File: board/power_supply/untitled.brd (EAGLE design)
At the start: 52 x 55 mm, 27 parts, among them IC1 317EMP, Q1 FDD4141TO252

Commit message: update boards 2022-07-14
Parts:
- C1: value (none) -> 22uF 25V
- C2: value (none) -> 10uF 10V
- C3, C4: value (none) -> 0.1uF
- R1: value (none) -> 300Ω
- R2: value (none) -> 470kΩ
- R3: value (none) -> 20kΩ
- R4: value (none) -> 1.2kΩ
- R6: value (none) -> 1.2KΩ 1/6W
- R7: value 10k -> 300Ω
- U$2: value SMD-R-TRIM -> 2.2kΩ
- U$4: value R-TRIM -> 20kΩ
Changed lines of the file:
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@@
 <?xml version="1.0" encoding="utf-8"?>
 <!DOCTYPE eagle SYSTEM "eagle.dtd">
-<eagle version="9.6.1">
+<eagle version="9.6.2">
 <drawing>
 <settings>
-<setting alwaysvectorfont="yes"/>
+<setting alwaysvectorfont="no"/>
 <setting verticaltext="up"/>
 </settings>
@@
 </layers>
 <board>
-<fusionsync huburn="a.cGVyc29uYWw6dWUyYjhiNWJj" projecturn="a.cGVyc29uYWw6dWUyYjhiNWJjIzIwMjIwNDE2NTE3MzEzNjU2" f3durn="urn:adsk.wipprod:dm.lineage:QmnGeXTNRAeKhx4INCeYVg" pcbguid="" lastpulledtime="" lastsyncedchangeguid="" latestrevisionid="b83a574e-0160-4f8e-8456-9f8577d503a8" lastsyncedrevisionid="b83a574e-0160-4f8e-8456-9f8577d503a8" lastboardhashguid="a0df0de1-b480-8f0f-8af4-34f871867293" lastpushedtime="2022-07-09T12:07:00Z" linktopcb3d="%12"/>
+<fusionsync huburn="a.cGVyc29uYWw6dWUyYjhiNWJj" projecturn="a.cGVyc29uYWw6dWUyYjhiNWJjIzIwMjIwNDE2NTE3MzEzNjU2" f3durn="urn:adsk.wipprod:dm.lineage:QmnGeXTNRAeKhx4INCeYVg" pcbguid="" lastpulledtime="" lastsyncedchangeguid="" latestrevisionid="b83a574e-0160-4f8e-8456-9f8577d503a8" lastsyncedrevisionid="b83a574e-0160-4f8e-8456-9f8577d503a8" lastboardhashguid="a0df0de1-b480-8f0f-8af4-34f871867293" lastpushedtime="2022-07-09T12:07:00Z" linktopcb3d="true"/>
 <plain>
 <wire x1="51.943" y1="-2.254" x2="51.943" y2="48.746" width="0.001" layer="20"/>
@@
 <attribute name="VALUE" x="3.81" y="12.63" size="0.0254" layer="27"/>
 </element>
-<element name="R1" library="adafruit" package="M2012" value="" x="31.75" y="15.748" smashed="yes">
+<element name="R1" library="adafruit" package="M2012" value="300Ω" x="31.75" y="15.748" smashed="yes">
 <attribute name="NAME" x="27.432" y="15.24" size="1.27" layer="25"/>
 <attribute name="VALUE" x="30.734" y="13.462" size="1.27" layer="27"/>
 </element>
-<element name="U$2" library="by_hirame" package="SMD-R-TRIM" value="SMD-R-TRIM" x="31.75" y="19.05" smashed="yes"/>
+<element name="U$2" library="by_hirame" package="SMD-R-TRIM" value="2.2kΩ" x="31.75" y="19.05" smashed="yes"/>
 <element name="MD1" library="Rembrandt Electronics - JST XH Connectors v1-0" package="JST-XH-02-PACKAGE-LONG-PAD" value="JST-XH-02-PIN-LONG-PAD" x="46.101" y="22.098" smashed="yes" rot="R270">
 <attribute name="NAME" x="43.37" y="20.82" size="1.016" layer="25" ratio="10" rot="R90"/>
@@
 <attribute name="PURCHASE-URL" value="https://pricing.snapeda.com/search/part/OKL-T/6-W12P-C/?ref=eda" x="21.209" y="37.846" size="1.778" layer="27" rot="R180" display="off"/>
 </element>
-<element name="R3" library="adafruit" package="M2012" value="" x="20.955" y="30.226" smashed="yes">
+<element name="R3" library="adafruit" package="M2012" value="20kΩ" x="20.955" y="30.226" smashed="yes">
 <attribute name="NAME" x="22.987" y="29.591" size="1.27" layer="25"/>
 <attribute name="VALUE" x="19.939" y="27.94" size="1.27" layer="27"/>
 </element>
-<element name="C1" library="adafruit" package="C2012" value="" x="20.955" y="28.067" smashed="yes" rot="R180">
+<element name="C1" library="adafruit" package="C2012" value="22uF 25V" x="20.955" y="28.067" smashed="yes" rot="R180">
 <attribute name="NAME" x="25.4" y="28.702" size="1.27" layer="25" rot="R180"/>
 <attribute name="VALUE" x="21.844" y="30.353" size="1.27" layer="27" rot="R180"/>
 </element>
-<element name="R4" library="adafruit" package="M2012" value="" x="8.255" y="30.226" smashed="yes">
+<element name="R4" library="adafruit" package="M2012" value="1.2kΩ" x="8.255" y="30.226" smashed="yes">
 <attribute name="NAME" x="7.239" y="27.813" size="1.27" layer="25"/>
 <attribute name="VALUE" x="7.239" y="27.94" size="1.27" layer="27"/>
 </element>
-<element name="C2" library="adafruit" package="C2012" value="" x="13.589" y="27.94" smashed="yes">
+<element name="C2" library="adafruit" package="C2012" value="10uF 10V" x="13.589" y="27.94" smashed="yes">
 <attribute name="NAME" x="15.748" y="27.305" size="1.27" layer="25"/>
 <attribute name="VALUE" x="12.7" y="25.654" size="1.27" layer="27"/>
 </element>
-<element name="R6" library="adafruit" package="0805-THM" value="" x="12.7" y="35.56" smashed="yes" rot="R270">
+<element name="R6" library="adafruit" package="0805-THM" value="1.2KΩ  1/6W" x="12.7" y="35.56" smashed="yes" rot="R270">
 <attribute name="NAME" x="14.224" y="38.608" size="1.27" layer="25" ratio="10" rot="R270"/>
 <attribute name="VALUE" x="9.925" y="38.6906" size="1.27" layer="27" ratio="10" rot="R270"/>
@@
 <attribute name="VALUE" x="24.13" y="7.6708" size="1.27" layer="27" rot="R180"/>
 </element>
-<element name="C3" library="generic" package="SMD1608" value="" x="21.59" y="11.684" smashed="yes">
+<element name="C3" library="generic" package="SMD1608" value="0.1uF" x="21.59" y="11.684" smashed="yes">
 <attribute name="NAME" x="20.79" y="12.334" size="1.016" layer="25"/>
 <attribute name="VALUE" x="20.79" y="10.034" size="1.016" layer="27"/>
 </element>
-<element name="C4" library="generic" package="SMD1608" value="" x="25.146" y="2.413" smashed="yes">
+<element name="C4" library="generic" package="SMD1608" value="0.1uF" x="25.146" y="2.413" smashed="yes">
 <attribute name="NAME" x="24.346" y="3.063" size="1.016" layer="25"/>
 <attribute name="VALUE" x="24.346" y="0.763" size="1.016" layer="27"/>
 </element>
-<element name="R2" library="adafruit" package="M2012" value="" x="31.75" y="13.462" smashed="yes" rot="R180">
+<element name="R2" library="adafruit" package="M2012" value="470kΩ" x="31.75" y="13.462" smashed="yes" rot="R180">
 <attribute name="NAME" x="29.718" y="14.097" size="1.27" layer="25" rot="R180"/>
 <attribute name="VALUE" x="32.766" y="15.748" size="1.27" layer="27" rot="R180"/>
 </element>
-<element name="U$4" library="by_hirame" package="R-TRIM" value="R-TRIM" x="8.128" y="36.703" smashed="yes" rot="R270"/>
+<element name="U$4" library="by_hirame" package="R-TRIM" value="20kΩ" x="8.128" y="36.703" smashed="yes" rot="R270"/>
 <element name="R5" library="adafruit" package="M2012" value="10k" x="28.448" y="10.033" smashed="yes" rot="R180">
 <attribute name="NAME" x="29.464" y="9.017" size="1.27" layer="25" rot="R180"/>
 <attribute name="VALUE" x="29.464" y="12.319" size="1.27" layer="27" rot="R180"/>
 </element>
-<element name="R7" library="adafruit" package="M2012" value="10k" x="28.448" y="5.08" smashed="yes">
+<element name="R7" library="adafruit" package="M2012" value="300Ω" x="28.448" y="5.08" smashed="yes">
 <attribute name="NAME" x="27.432" y="6.096" size="1.27" layer="25"/>
 <attribute name="VALUE" x="27.432" y="2.794" size="1.27" layer="27"/>

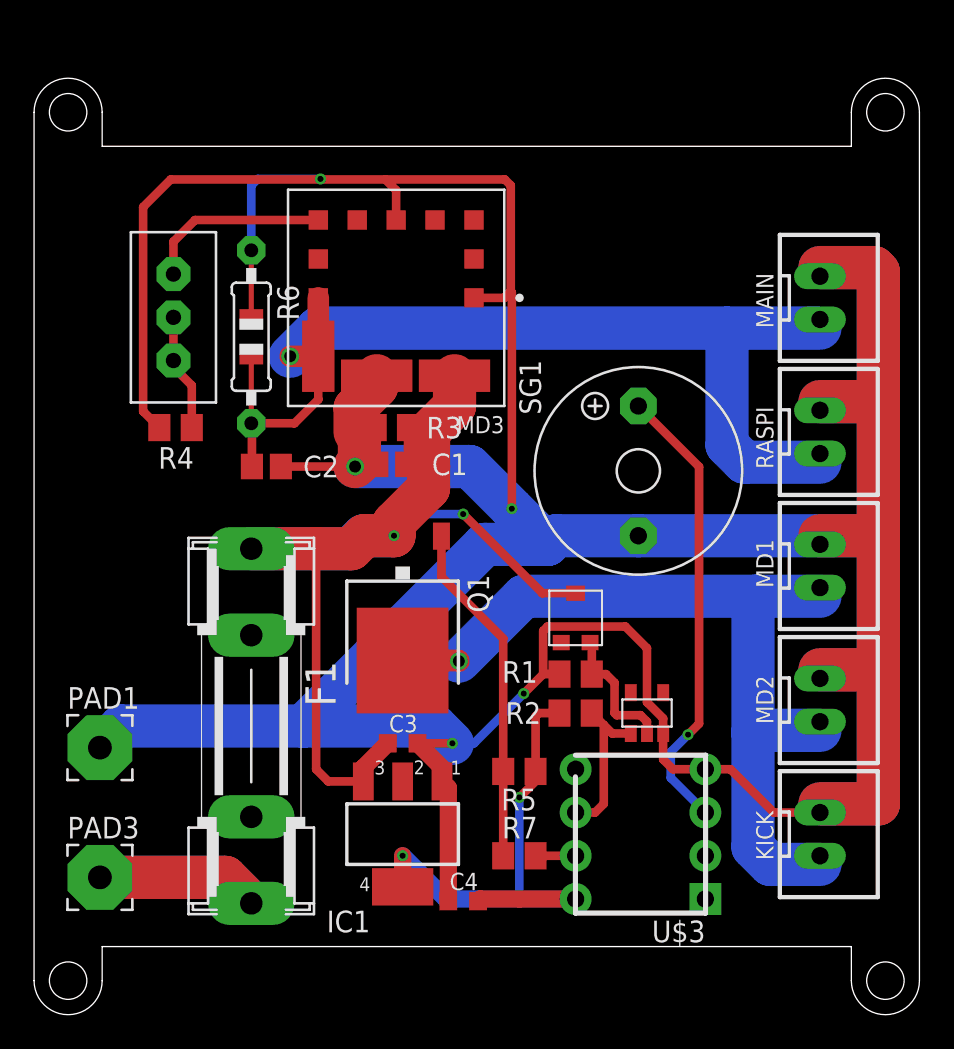
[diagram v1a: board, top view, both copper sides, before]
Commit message: marge前のファイル
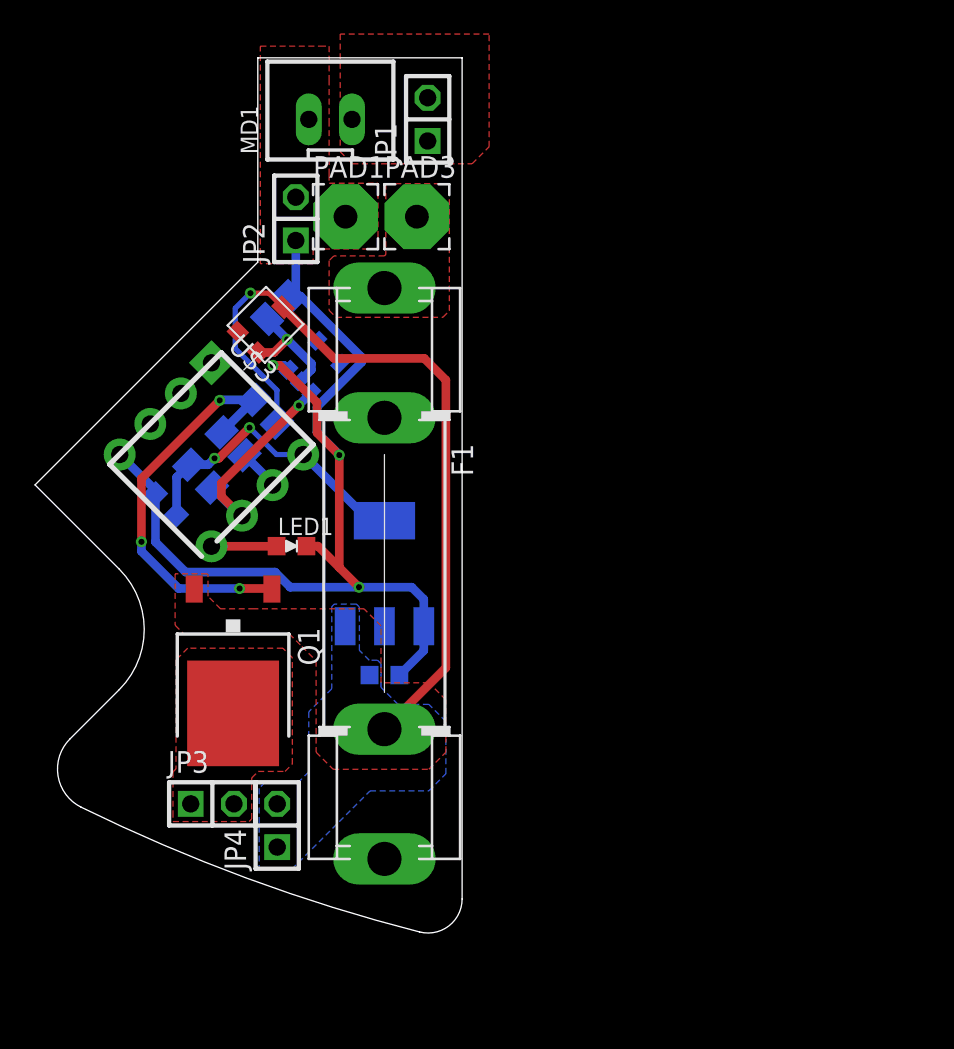
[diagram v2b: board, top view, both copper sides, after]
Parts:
- removed C1: 22uF 25V, adafruit:C2012
- removed C2: 10uF 10V, adafruit:C2012
- removed KICK, MAIN, MD2, RASPI: JST-XH-02-PIN-LONG-PAD, Rembrandt Electronics - JST XH Connectors v1-0:JST-XH-02-PACKAGE-LONG-PAD
- removed MD3: OKL-T/6-W12P-CMURATA_OKL-T-6-W12P-C_0_0, OKL-T_6-W12P-C:MURATA_OKL-T-6-W12P-C_0
- removed R3: 20kΩ, adafruit:M2012
- removed R4: 1.2kΩ, adafruit:M2012
- removed R6: 1.2KΩ 1/6W, adafruit:0805-THM
- removed SG1: F/TMB, buzzer:F/TMB
- removed U$4: 20kΩ, by_hirame:R-TRIM
- added JP1, JP2, JP3, JP4: (no value), pinhead:1X02
- added LED1: LED1608, generic:LED1608
- F1: device fuse:SHK20L -> fuse:SH32
- moved PAD3 43.0 mm to (22.4, 42.6)
- moved MD1 38.9 mm to (17.3, 48.3), turned to 0 degrees
- moved PAD1 34.4 mm to (18.2, 42.6)
- moved U$3 33.6 mm to (10.4, 28.6), turned to 315 degrees
- moved R7 29.5 mm to (11.6, 29.3), flipped to the bottom, turned to 225 degrees
- moved C4 29.1 mm to (7.69, 25.7), flipped to the bottom, turned to 225 degrees
- moved U$1 28.2 mm to (16.4, 33.8), flipped to the bottom, turned to 45 degrees
- moved R1 27.7 mm to (14.3, 37.3), flipped to the bottom, turned to 315 degrees
- moved R2 26.1 mm to (9.73, 27.4), flipped to the bottom, turned to 45 degrees
- moved R5 25.9 mm to (13.5, 31.2), flipped to the bottom, turned to 45 degrees
- moved U$2 25.1 mm to (13.5, 36.3), turned to 315 degrees
- moved IC1 15.3 mm to (20.5, 21.7), flipped to the bottom, turned to 0 degrees
- moved F1 11.9 mm to (20.5, 21.7)
- moved Q1 10.4 mm to (11.6, 15.9)
- moved C3 4.15 mm to (20.5, 15.7), flipped to the bottom, turned to 180 degrees
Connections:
- removed net N$8: C2.1, MAIN.2, MD3.4, MD3.5, R6.2, RASPI.2
- removed net N$9: MD3.6, U$4.P$1
- net GND: now also JP2.1, JP2.2, LED1.K; no longer C1.2, C2.2, KICK.1, MAIN.1, MD2.1, MD3.1, MD3.3, MD3.7, R3.1, R4.1, R6.1, RASPI.1, SG1.-
- net N$11: no longer R5.1
- net N$3: now also F1.1A; no longer F1.2A
- net N$5: now also JP3.1, JP3.2; no longer KICK.2, MD1.2, MD2.2
- net N$6: now also LED1.A, U$3.5; no longer SG1.+, U$3.3
- net N$7: now also JP1.1, JP1.2, MD1.2; no longer R4.2, U$4.P$2, U$4.P$3
- net VCC: now also F1.2A, JP4.1, JP4.2, R5.1; no longer C1.1, F1.1A, MD3.2, R3.2
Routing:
- net GND: track 301.2 -> 63.5 mm, vias 5 -> 3
- net N$8: track 60.2 -> 0.00 mm, vias 1 -> 0
- net N$5: track 50.8 -> 0.00 mm, vias 1 -> 0
- net N$6: track 26.9 -> 3.83 mm, vias 1 -> 0
- net VCC: track 66.2 -> 44.6 mm, vias 2 -> 1
- net N$3: track 19.0 -> 0.00 mm
- net N$11: track 31.4 -> 17.9 mm
- net N$9: track 10.9 -> 0.00 mm
- net N$7: track 6.92 -> 0.00 mm
- net N$2: track 20.3 -> 24.1 mm, vias 0 -> 3
- net N$4: track 9.28 -> 12.4 mm, vias 0 -> 1
- net N$1: track 8.03 -> 7.03 mm, vias 0 -> 1
- added copper zone on layer 1, net GND
- added copper zone on layer 1, net N$3
- added copper zone on layer 1, net N$5
- added copper zone on layer 1, net N$7
- added copper zone on layer 1, net VCC
- added copper zone on layer 16, net VCC
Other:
- board size 52 x 55 mm -> 25.1 x 51.4 mm
